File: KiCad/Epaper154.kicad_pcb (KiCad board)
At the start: 2 copper layers, 58.2 x 37 mm, 30 parts, among them J1 USB-C, J2 DC, J3 TEMP, U1 LMR16006+FB, U2 FT231XQ, U3 ESP32-PICO-MINI-02, U4 QR

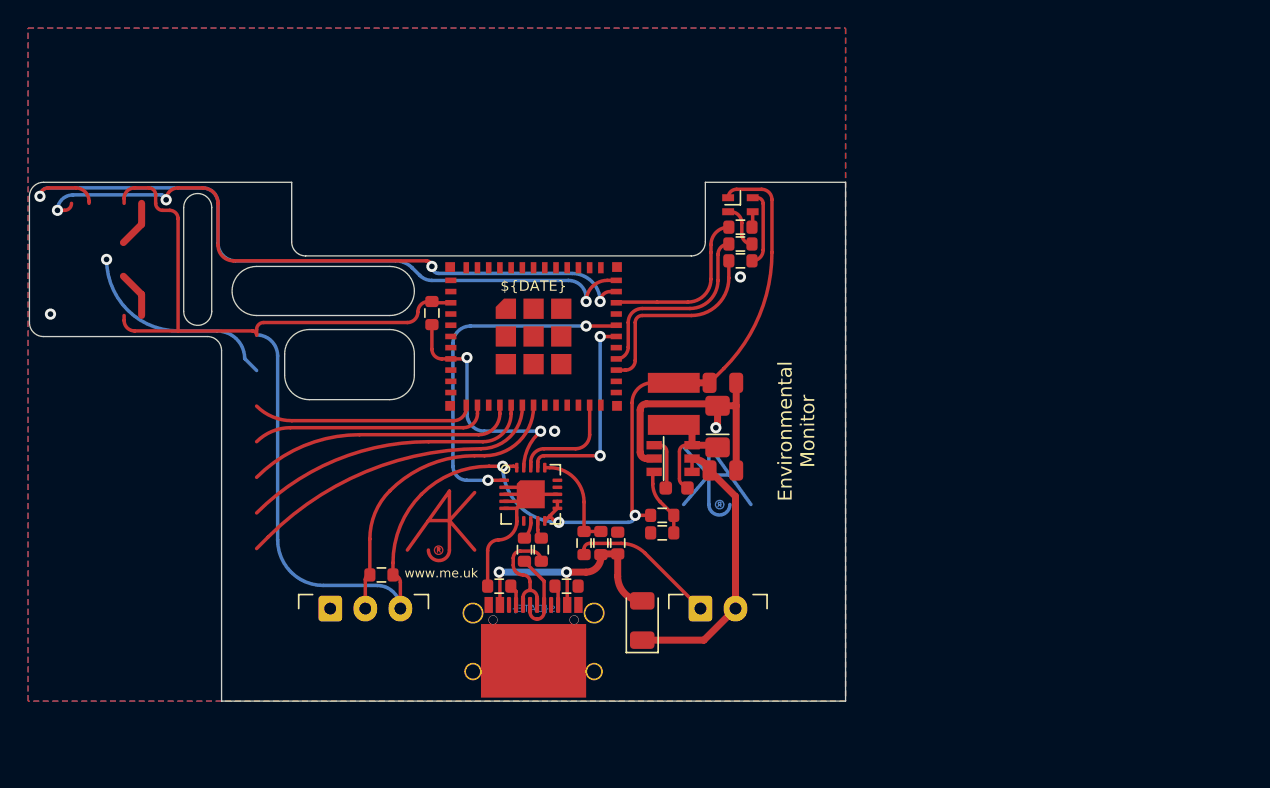
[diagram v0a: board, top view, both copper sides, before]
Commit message: Started
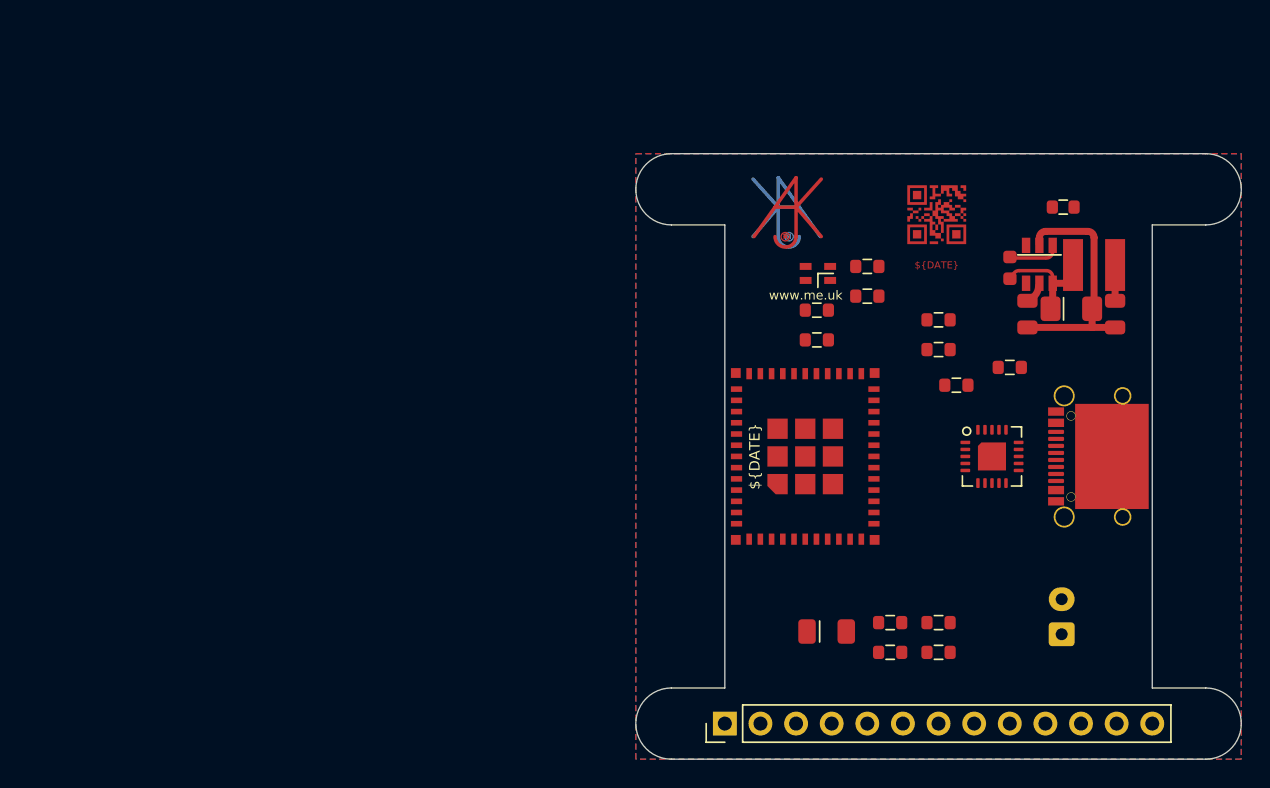
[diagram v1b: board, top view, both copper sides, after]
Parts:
- removed J3: TEMP, RevK:Molex_MiniSPOX_H3RA
- removed R10: 4k7, RevK:R_0603
- added M1: EPaper, Connector_PinHeader_2.54mm:PinHeader_1x13_P2.54mm_Vertical, F.Cu at (135.9, 101.6)
- D2: footprint Diode_SMD:D_1206_3216Metric -> RevK:D_1206
- U4: footprint RevK:QR-ENVMON -> RevK:QR-GFX; moved to F.Cu
- moved J1 47.4 mm to (166.4, 82.5), turned to 90 degrees
- moved U4 42.8 mm to (151.0, 65.3)
- moved C4 39.8 mm to (160.0, 64.8), turned to 0 degrees
- moved R5 35.9 mm to (156.2, 76.2), turned to 0 degrees
- moved R3 35.6 mm to (152.4, 77.5), turned to 0 degrees
- moved Logo2 33.3 mm to (141.0, 64.8)
- moved U2 33.0 mm to (154.9, 82.5)
- moved R9 31.1 mm to (146.1, 71.1), turned to 0 degrees
- moved R13 30.5 mm to (151.1, 94.4), turned to 0 degrees
- moved R11 29.9 mm to (147.7, 96.5), turned to 0 degrees
- moved U1 29.6 mm to (158.3, 68.8), turned to 0 degrees
- moved R7 27.8 mm to (151.1, 74.9), turned to 0 degrees
- moved R8 26.5 mm to (151.1, 96.5), turned to 0 degrees
- moved R6 25.7 mm to (142.4, 74.2), turned to 0 degrees
- moved R2 24.9 mm to (151.1, 72.8)
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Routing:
- net +3V3: track 128.4 -> 0.00 mm, vias 3 -> 0
- net unconnected-(U3-Pad35): track 52.1 -> 0.00 mm, vias 2 -> 0
- net GND: track 50.1 -> 0.00 mm, vias 5 -> 0
- net unconnected-(U3-Pad34): track 48.4 -> 0.00 mm, vias 4 -> 0
- net O: track 25.3 -> 0.00 mm, vias 2 -> 0
- net unconnected-(U3-Pad17): track 22.6 -> 0.00 mm
- net TEMP: track 21.8 -> 0.00 mm
- net unconnected-(U3-Pad16): track 21.1 -> 0.00 mm
- net unconnected-(U3-Pad15): track 19.6 -> 0.00 mm
- net DC: track 19.1 -> 0.00 mm
- net VBUS: track 18.3 -> 0.00 mm, vias 2 -> 0
- net EN: track 17.5 -> 0.00 mm, vias 2 -> 0
- net unconnected-(U3-Pad13): track 17.2 -> 0.00 mm
- net unconnected-(U3-Pad12): track 15.9 -> 0.00 mm
- net I: track 14.8 -> 0.00 mm, vias 2 -> 0
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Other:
- board size 58.2 x 37 mm -> 43.2 x 43.2 mm
- board text removed: "14"
- board text removed: "25"
- board text removed: "26"
- board text removed: "27"
- board text removed: "3.3"
- board text removed: "32"
- board text removed: "33"
- board text removed: "CO₂"
- board text removed: "DC 4V-60V"
- board text removed: "DS18B20"
- board text removed: "Environmental Monitor"
- board text removed: "LED: 7/19/8"
- board text removed: "SCD41 SCL: 21 SDA: 22"
- board text removed: "⏚"
